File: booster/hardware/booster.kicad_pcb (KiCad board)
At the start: 2 copper layers, 31.1 x 14 mm, 5 parts, among them J1 12V_booster, J4 Conn_01x03, U1 LM2940IMP-10/NOPB

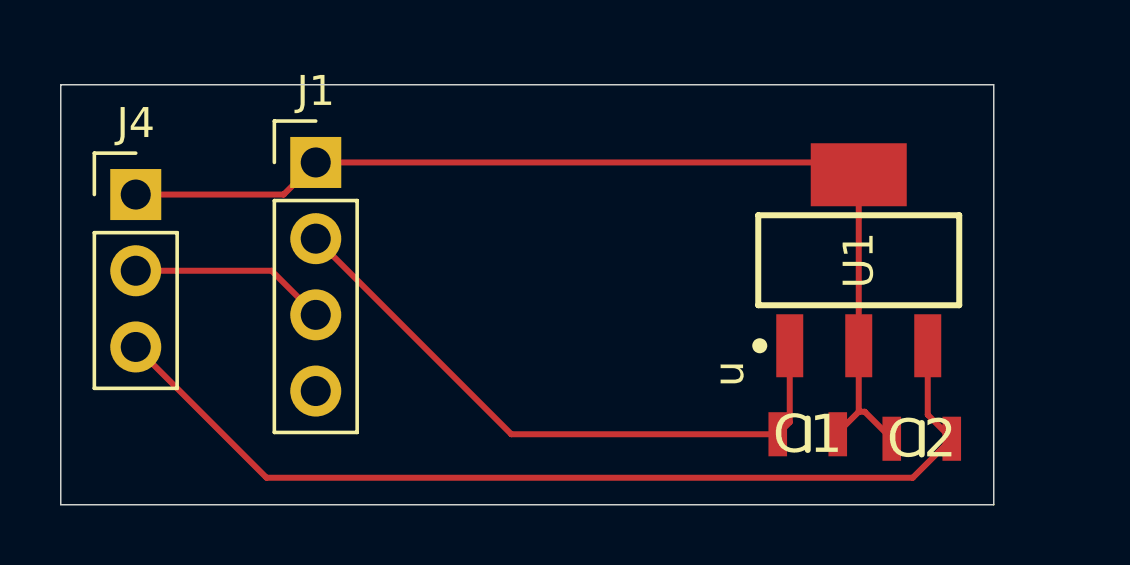
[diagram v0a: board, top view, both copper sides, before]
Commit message: made booster board pcb
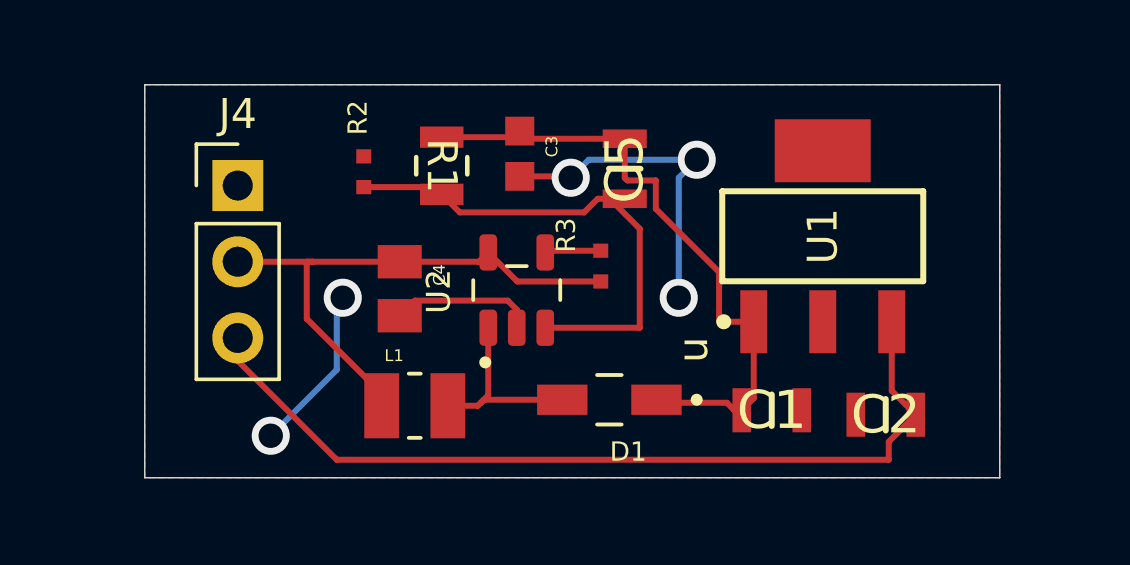
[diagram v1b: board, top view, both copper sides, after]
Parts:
- removed J1: 12V_booster, Connector_PinHeader_2.54mm:PinHeader_1x04_P2.54mm_Vertical
- added C3: 10uF, booster:smd_cap_10uf_16V, F.Cu at (134.3, 87.5)
- added C4: 22uF, booster:smd_cap_22uf_16V, F.Cu at (130.3, 92.0)
- added C5: 22pF, booster:CAPC2012X145N, F.Cu at (137.8, 88.0)
- added D1: MBR120VLSFT1G, booster:MBR120VLSFT1G, F.Cu at (137.3, 95.7)
- added L1: MLP2520S100MT0S1, booster:INDC10uh, F.Cu at (130.8, 95.9)
- added R1: 876k, booster:smd_res_876k_KOA, F.Cu at (131.7, 87.9)
- added R2: 100k, booster:smd_res_100k, F.Cu at (129.1, 88.1)
- added R3: 100k, booster:smd_res_100k, F.Cu at (137.0, 91.2)
- added U2: TPS61040DBVR, booster:TPS61040DBVR, F.Cu at (134.2, 92.0)
- moved J4 3.41 mm to (124.9, 88.6)
- moved C1 1.44 mm to (142.7, 96.1)
- moved C2 1.44 mm to (146.5, 96.2)
- moved U1 1.44 mm to (144.4, 90.3)
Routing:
- net Net-(U2-FB): track 0.00 -> 16.6 mm
- net GND: track 35.4 -> 21.8 mm, vias 0 -> 5
- net /5V: track 6.61 -> 19.2 mm
- net Net-(U2-SW): track 0.00 -> 6.50 mm
- net /10V: track 33.0 -> 29.1 mm
- net Net-(U2-EN): track 0.00 -> 1.87 mm
- added copper zone on F.Cu, net GND
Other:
- board size 31.1 x 14 mm -> 28.5 x 13.1 mm

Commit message: made whole pcb
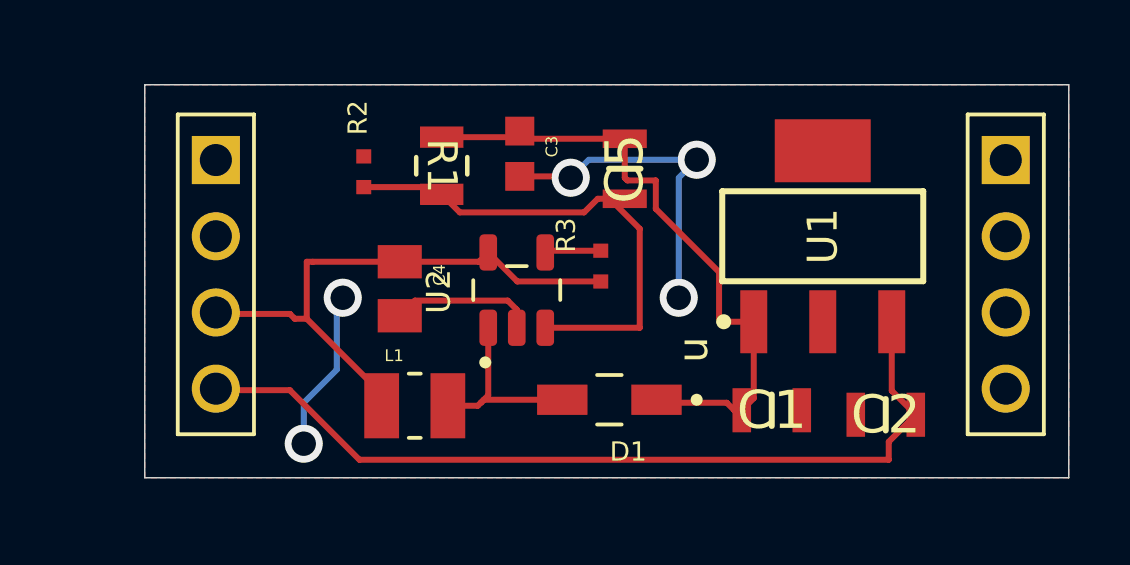
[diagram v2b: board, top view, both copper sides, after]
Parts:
- removed J4: Conn_01x03, Connector_PinHeader_2.54mm:PinHeader_1x03_P2.54mm_Vertical
- added J1: i/o, booster:board headers, F.Cu at (121.8, 85.0)
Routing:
- net /10V: track 29.1 -> 28.4 mm
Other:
- board size 28.5 x 13.1 mm -> 30.8 x 13.1 mm
